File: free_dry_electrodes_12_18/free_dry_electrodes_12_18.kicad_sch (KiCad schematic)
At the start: 30 parts

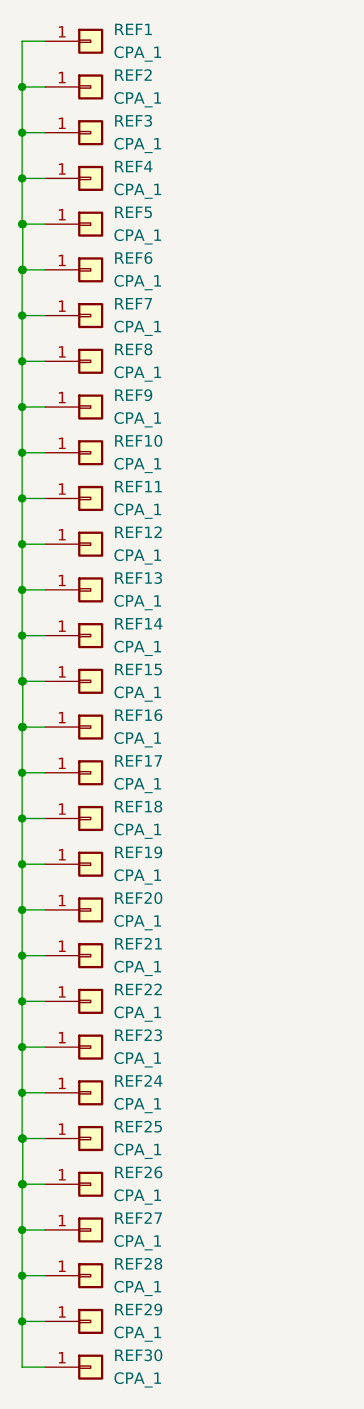
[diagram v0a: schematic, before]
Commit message: Add files via upload
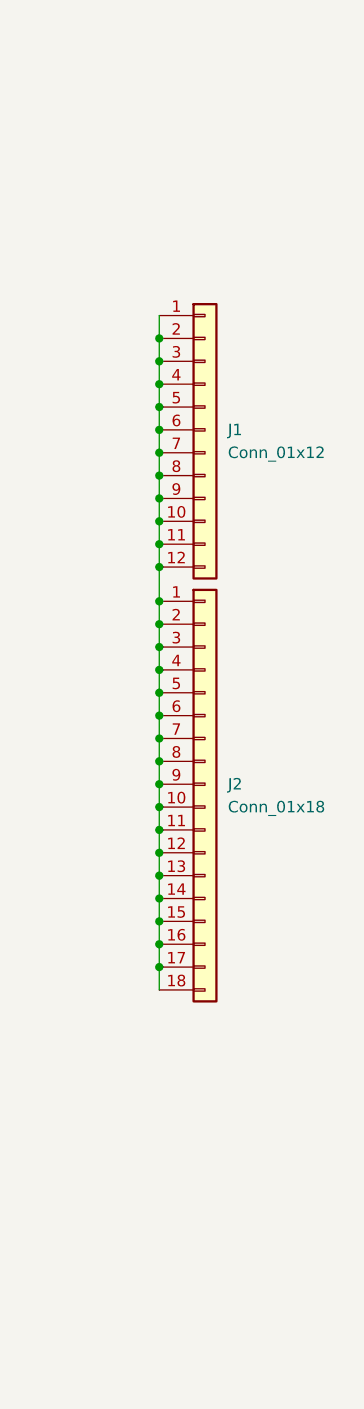
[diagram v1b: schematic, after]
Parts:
- removed REF1: CPA_1, symbol Connector_Generic:Conn_01x01
- removed REF10, REF11, REF12, REF13, REF14, REF15, REF16, REF17, REF18, REF19, REF2, REF20, REF21, REF22, REF23, REF24, REF25, REF26, REF27, REF28, REF29, REF3, REF30, REF4, REF5, REF6, REF7, REF8, REF9: CPA_1, 1024_dry_electrodes:CPA_1, symbol Connector_Generic:Conn_01x01
- added J1: Conn_01x12, 1024_dry_electrodes:CPA_12, symbol Connector_Generic:Conn_01x12
- added J2: Conn_01x18, 1024_dry_electrodes:CPA_18, symbol Connector_Generic:Conn_01x18
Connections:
- new net: J1.1 (Pin_1), J1.10 (Pin_10), J1.11 (Pin_11), J1.12 (Pin_12), J1.2 (Pin_2), J1.3 (Pin_3), J1.4 (Pin_4), J1.5 (Pin_5), J1.6 (Pin_6), J1.7 (Pin_7), J1.8 (Pin_8), J1.9 (Pin_9), J2.1 (Pin_1), J2.10 (Pin_10), J2.11 (Pin_11), J2.12 (Pin_12), J2.13 (Pin_13), J2.14 (Pin_14), J2.15 (Pin_15), J2.16 (Pin_16), J2.17 (Pin_17), J2.18 (Pin_18), J2.2 (Pin_2), J2.3 (Pin_3), J2.4 (Pin_4), J2.5 (Pin_5), J2.6 (Pin_6), J2.7 (Pin_7), J2.8 (Pin_8), J2.9 (Pin_9)
